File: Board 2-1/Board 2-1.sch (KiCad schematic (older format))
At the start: 50 parts, among them J1 FROM PULSE WIDTH SLIDER, J2 SAWTOOTH FROM VCO-2, J3 PULSE WAVE OUTPUT, J4 POSITIVE SUPPLY, J5 GND, J6 NEGATIVE SUPPLY, J7 PULSE WIDTH MOD IN, J8 SINE WAVE OUTPUT, J9 TRIANGLE WAVE OUT, Q1 2N3906, Q2 2N5172, Q3-1 2SK30, Q3-2 2SK30

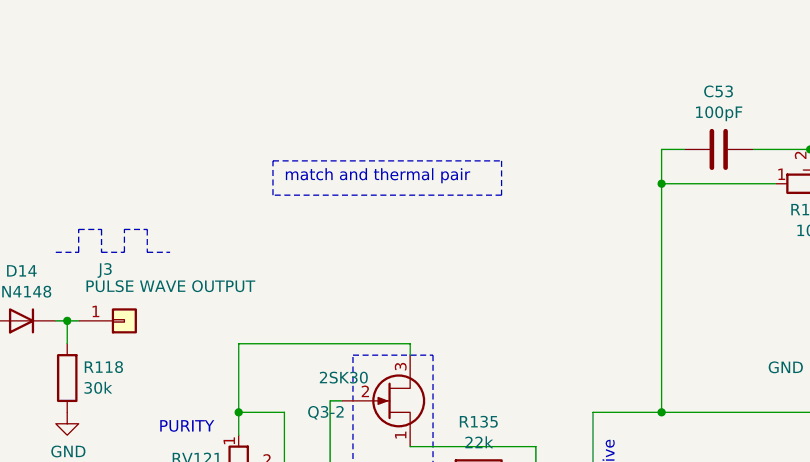
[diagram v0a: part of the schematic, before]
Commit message: various fixes
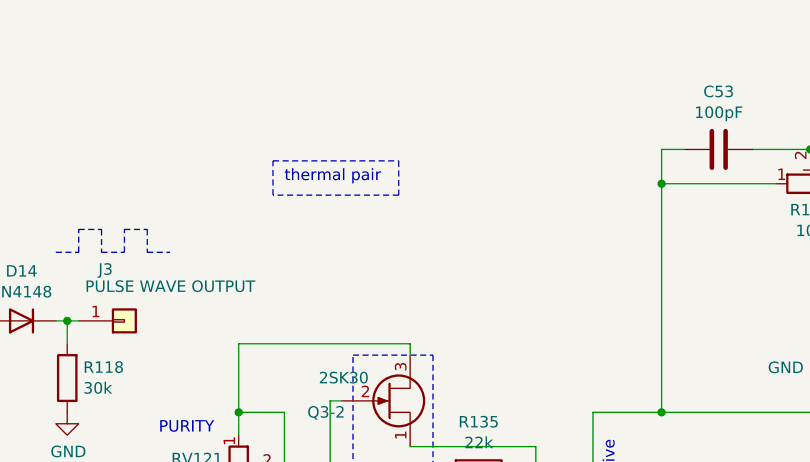
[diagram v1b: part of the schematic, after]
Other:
- note added: "thermal pair"
- note removed: "match and thermal pair"
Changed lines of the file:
@@
 	6900 1900 6900 1950
 Text Notes 6350 1200 0    50   ~ 0
-match and thermal pair
+thermal pair
 Wire Notes Line
-	6300 1100 7300 1100
+	6300 1100 6850 1100
 Wire Notes Line
-	7300 1100 7300 1250
+	6850 1100 6850 1250
 Wire Notes Line
-	7300 1250 6300 1250
+	6850 1250 6300 1250
 Wire Notes Line
 	6300 1250 6300 1100
